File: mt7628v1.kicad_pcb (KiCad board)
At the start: 4 copper layers, 62 x 50.1 mm, 142 parts, among them U1 W9725G6KB-25, U3 W25Q32JVSS, Y1 Crystal_40Mhz

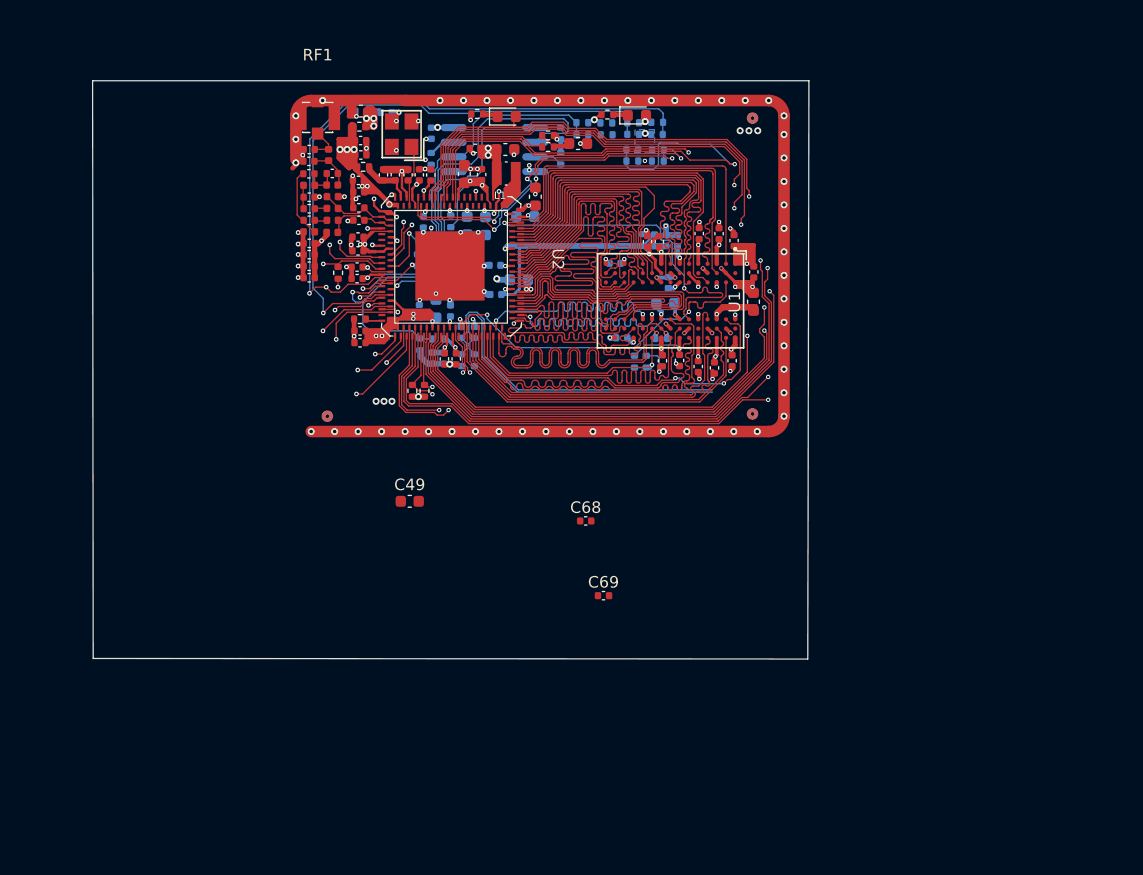
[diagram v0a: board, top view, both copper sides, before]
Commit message: final_all_router by asif
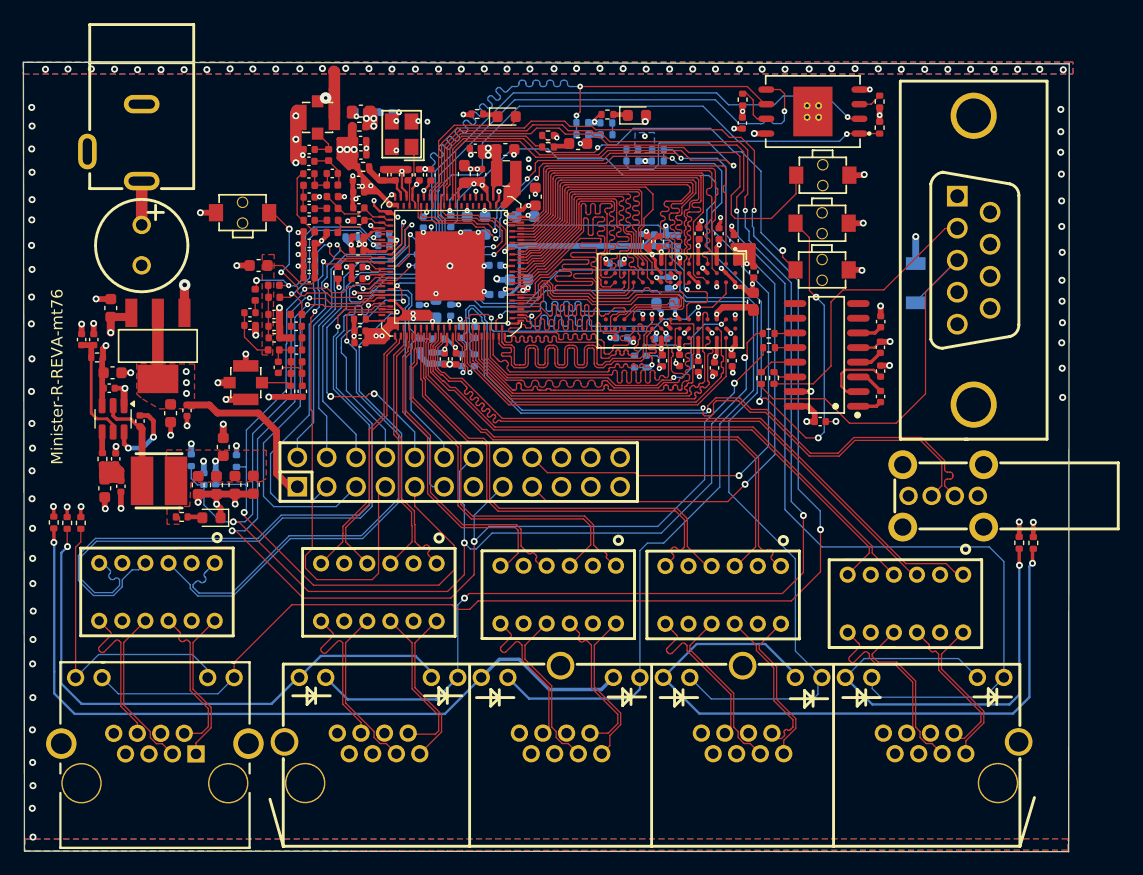
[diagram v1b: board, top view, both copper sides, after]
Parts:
- removed ? (x14): , 
- removed C68: 1uf/6.3v, Capacitor_SMD:C_0402_1005Metric
- removed R15, R16: 10K/1% NC, Resistor_SMD:R_0402_1005Metric
- added C100: 10pf/50v, Capacitor_SMD:C_0402_1005Metric, F.Cu at (117.6, 111.2)
- added C101: 10pf/50v, Capacitor_SMD:C_0402_1005Metric, F.Cu at (113.6, 110.1)
- added C102: 1.2pf/50v, Capacitor_SMD:C_0402_1005Metric, F.Cu at (113.6, 111.2)
- added C103: 1.2pf/50v, Capacitor_SMD:C_0402_1005Metric, F.Cu at (117.7, 113.3)
- added C104: 9pf/50v, Capacitor_SMD:C_0402_1005Metric, F.Cu at (116.1, 114.8)
- added C105: 1.8Pf/50v, Capacitor_SMD:C_0402_1005Metric, F.Cu at (118.2, 116.9)
- added C106: 1.8Pf/50v, Capacitor_SMD:C_0402_1005Metric, F.Cu at (117.1, 116.9)
- added C74: 22uf/25v, Capacitor_SMD:C_0603_1608Metric, F.Cu at (101.6, 109.7)
- added C75: 10uf/6.3v, Capacitor_SMD:C_0603_1608Metric, F.Cu at (106.8, 118.8)
- added C76: 100nf/16v, Capacitor_SMD:C_0402_1005Metric, F.Cu at (108.2, 118.5)
- added C78: 470uf/25v, easyeda2kicad:CAP-TH_BD8.0-P3.50-D0.6-FD, F.Cu at (104.2, 104.2)
- added C79: 2pf/50v, Capacitor_SMD:C_0402_1005Metric, B.Cu at (125.2, 104.3)
- added C80: 2pf/50v, Capacitor_SMD:C_0402_1005Metric, B.Cu at (125.2, 103.3)
- added C81: 1uf/6.3v, Capacitor_SMD:C_0402_1005Metric, F.Cu at (115.7, 112.2)
- added C82: 1uf/6.3v, Capacitor_SMD:C_0402_1005Metric, F.Cu at (115.7, 110.2)
- added C83: 100pf/50v, Capacitor_SMD:C_0402_1005Metric, F.Cu at (115.7, 111.2)
- added C84: 10uf/25v, Capacitor_SMD:C_0603_1608Metric, F.Cu at (101.7, 115.3)
- added C85: 100nf/16v, Capacitor_SMD:C_0402_1005Metric, F.Cu at (101.4, 116.6)
- added C86: NC, Capacitor_SMD:C_0402_1005Metric, F.Cu at (99.0, 112.4)
- added C87: NC, Capacitor_SMD:C_0402_1005Metric, F.Cu at (100.1, 112.4)
- added C88: 1uf/25v, Capacitor_SMD:C_0402_1005Metric, F.Cu at (104.1, 119.5)
- added C89: 22uf/25v, Capacitor_SMD:C_0603_1608Metric, F.Cu at (111.3, 121.7)
- added C90: 22uf/25v, Capacitor_SMD:C_0603_1608Metric, F.Cu at (113.9, 125.0)
- added C91: 22uf/25v, Capacitor_SMD:C_0603_1608Metric, F.Cu at (112.3, 125.0)
- added C92: 22uf/25v, Capacitor_SMD:C_0603_1608Metric, F.Cu at (110.7, 125.0)
- added C93: 22uf/25v, Capacitor_SMD:C_0603_1608Metric, F.Cu at (109.1, 125.0)
- added C94: NC, Capacitor_SMD:C_0402_1005Metric, F.Cu at (102.5, 125.1)
- added C95: 100nf/16v, Capacitor_SMD:C_0402_1005Metric, F.Cu at (168.2, 117.3)
- added C96: 100nf/16v, Capacitor_SMD:C_0402_1005Metric, F.Cu at (168.2, 113.1)
- added C97: 100nf/16v, Capacitor_SMD:C_0402_1005Metric, F.Cu at (168.2, 110.8)
- added C98: 100nf/16v, Capacitor_SMD:C_0402_1005Metric, F.Cu at (163.0, 119.5)
- added C99: 100nf/16v, Capacitor_SMD:C_0402_1005Metric, F.Cu at (168.2, 115.1)
- added D3: LED, Diode_SMD:D_0603_1608Metric, F.Cu at (110.3, 127.8)
- added D4: ZMM5V1, easyeda2kicad:LL-34_L3.5-W1.5-RD, B.Cu at (171.2, 107.5)
- added J1: Barrel_Jack_Switch, easyeda2kicad:DC-IN-TH_DC-005C-20A, F.Cu at (101.9, 95.4)
- added J2: DE9_Pins, easyeda2kicad:HDR-TH_HL-DP9HB180F, F.Cu at (176.3, 105.5)
- added J3: Conn_01x24_MountingPin, easyeda2kicad:HDR-TH_24P-P2.54-V-M-R2-C12-S2.54, F.Cu at (131.7, 123.9)
- added J4: RJ45_LED_Shielded_x2, easyeda2kicad:RJ45-TH_DS1128-09-S8B8X, F.Cu at (105.4, 145.0)
- added L10: 10nh, Inductor_SMD:L_0402_1005Metric, F.Cu at (115.7, 108.7)
- added L11: 6.8uh, easyeda2kicad:IND-SMD_L4.5-W4.0_GCD43-XX, F.Cu at (105.8, 124.6)
- added L12: 10nh, Inductor_SMD:L_0402_1005Metric, F.Cu at (115.7, 107.7)
- added L13: 2nh, Inductor_SMD:L_0402_1005Metric, F.Cu at (117.6, 110.2)
- added L14: 2nh, Inductor_SMD:L_0402_1005Metric, F.Cu at (114.1, 108.5)
- added L15: 2.7nh, Inductor_SMD:L_0402_1005Metric, F.Cu at (117.6, 112.2)
- added L16: 2.7nh, Inductor_SMD:L_0402_1005Metric, F.Cu at (115.7, 113.3)
- added L17: 1.2nh, Inductor_SMD:L_0402_1005Metric, F.Cu at (117.7, 114.3)
- added L18: 2nh, Inductor_SMD:L_0402_1005Metric, F.Cu at (117.6, 115.3)
- added R39: 510/0402, Resistor_SMD:R_0402_1005Metric, F.Cu at (107.7, 127.8)
- added R40: 1k/1%, Resistor_SMD:R_0402_1005Metric, F.Cu at (97.8, 128.3)
- added R41: 1k/1%, Resistor_SMD:R_0402_1005Metric, F.Cu at (96.6, 128.2)
- added R42: 1k/1%, Resistor_SMD:R_0402_1005Metric, F.Cu at (181.4, 130.0)
- added R43: 1k/1%, Resistor_SMD:R_0402_1005Metric, F.Cu at (180.2, 130.0)
- added R44: 1k/1%, Resistor_SMD:R_0402_1005Metric, F.Cu at (99.0, 128.3)
- added R46: 100K/0402, Resistor_SMD:R_0402_1005Metric, F.Cu at (100.4, 114.0)
- added R47: 1k/1%, Resistor_SMD:R_0402_1005Metric, F.Cu at (100.8, 122.7)
- added R48: 6.2K/0603, Capacitor_SMD:C_0603_1608Metric, F.Cu at (101.0, 125.3)
- added R49: 2K/0402, Capacitor_SMD:C_0402_1005Metric, F.Cu at (102.0, 122.7)
- added R50: 0, Resistor_SMD:R_0402_1005Metric, F.Cu at (158.5, 111.9)
- added R52: 0, Resistor_SMD:R_0402_1005Metric, F.Cu at (158.6, 113.1)
- added R55: 0, Resistor_SMD:R_0402_1005Metric, F.Cu at (157.9, 115.7)
- added R57: 0, Resistor_SMD:R_0402_1005Metric, F.Cu at (159.0, 115.7)
- added RF2: ANT_SHAFT_SEAT, easyeda2kicad:IPEX-SMD_4P-L2.6-W2.6_C9900016457, F.Cu at (113.3, 116.1)
- added SW_GPIO1: GPIO, easyeda2kicad:SW-SMD_L3.9-W2.9-LS4.8-EH-A, F.Cu at (113.0, 101.4)
- added SW_GPIO3: PORST, easyeda2kicad:SW-SMD_L3.9-W2.9-LS4.8-EH-A, F.Cu at (163.1, 106.4)
- added SW_REF_CLK1: REF_CLK, easyeda2kicad:SW-SMD_L3.9-W2.9-LS4.8-EH-A, F.Cu at (163.2, 98.2)
- added SW_WDT_RST1: WDT_RST, easyeda2kicad:SW-SMD_L3.9-W2.9-LS4.8-EH-A, F.Cu at (163.1, 102.3)
- added U10: ~, easyeda2kicad:RJ45-TH_B-1-4, F.Cu at (148.4, 144.4)
- added U11: TF-1016DG-LAN3, easyeda2kicad:DIP-12_L12.8-W7.3-P2.00-LS5.0-BL, F.Cu at (140.3, 134.5)
- added U12: TF-1016DG-LAN2, easyeda2kicad:DIP-12_L12.8-W7.3-P2.00-LS5.0-BL, F.Cu at (154.6, 134.5)
- added U13: TF-1016DG-LAN1, easyeda2kicad:DIP-12_L12.8-W7.3-P2.00-LS5.0-BL, F.Cu at (170.3, 135.2)
- added U14: TF-1016DG-WAN, easyeda2kicad:DIP-12_L12.8-W7.3-P2.00-LS5.0-BL, F.Cu at (105.6, 134.2)
- added U4: ams1117-5v, easyeda2kicad:SOT-223_L6.5-W3.5-P2.30-LS7.0-BR, F.Cu at (105.7, 113.0)
- added U6: TF-1016DG-LAN4, easyeda2kicad:DIP-12_L12.8-W7.3-P2.00-LS5.0-BL, F.Cu at (124.8, 134.3)
- added U7: MP1470, Package_TO_SOT_SMD:TSOT-23-6, F.Cu at (101.8, 119.3)
- added U8: SP3232, easyeda2kicad:SOIC-16_L9.9-W3.9-P1.27-LS6.0-BL, F.Cu at (163.5, 113.7)
- added U9: USB_VERTICLE, easyeda2kicad:USB-A-TH_USB-226-BRW, F.Cu at (173.6, 125.9)
- C69: moved to B.Cu
- C70, R22, R23, R24: moved to F.Cu
- L1: value 2.2 uH/VLS252012T-2R2M1R3 -> 2.2 uH/VLS252012ET-2R2M; footprint Library:IND_VLS252012ET-100M -> easyeda2kicad:IND-SMD_L2.5-W2.0_VLS2520X
- U1: value W9725G6KB-25 -> W971GG6SB25I; footprint easyeda2kicad:WBGA-84_L12.5-W8.0-P0.80-TL_WINBOND_W9725G6KB -> easyeda2kicad:WBGA-84_L12.5-W8.0-P0.80-TL_W9751G6KB
- U2: value ~ -> MT7628NN
- U3: value W25Q32JVSS -> W25Q256JVEIQ; footprint easyeda2kicad:SOIC-8_L5.3-W5.3-P1.27-LS8.0-BL -> easyeda2kicad:WSON-8_L8.0-W6.10-P1.27-BL-EP; moved to F.Cu
- moved R5 48.4 mm to (110.7, 124.4), turned to -90 degrees
- moved R29 48.1 mm to (108.5, 122.8), turned to -90 degrees
- moved R28 47.7 mm to (109.6, 124.5), turned to -90 degrees
- moved R6 46.7 mm to (112.5, 122.9), turned to -90 degrees
- moved C69 38.0 mm to (122.4, 103.5), turned to 180 degrees
- moved R22 28.0 mm to (168.1, 91.8), turned to 90 degrees
- moved U3 27.8 mm to (162.3, 92.7), turned to 90 degrees
- moved R23 27.6 mm to (168.1, 94.1), turned to 90 degrees
- moved R24 27.4 mm to (156.3, 91.6)
- moved C70 26.9 mm to (156.2, 93.7)
- moved C49 24.2 mm to (114.4, 106.0), turned to 180 degrees
- moved R17 0.06 mm to (131.0, 109.9)
- moved C32 0.05 mm to (134.0, 102.5)
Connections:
- net Net-(U2C-WDT_RST_N) renamed WDT_RST
- net Net-(U2D-USB_DM) renamed USB_DP-
- net Net-(U2D-USB_DP) renamed USB_DP+
- U1 pad R8: MADDR13 -> unconnected-(U1-A13(2GB)-PadR8)
- U2 pad 11: unconnected-(U2A-WF1_RFION-Pad11) -> WF1_RF1ON
- U2 pad 12: unconnected-(U2A-WF1_RFIOP-Pad12) -> WF1_RF1OP
- U2 pad 138: PORST_N -> CPURST_N
- U2 pad 139: WIFI_RESET -> LINK4
- U2 pad 140: unconnected-(U2E-AVDD33_TX_P1234_2-Pad140) -> LINK3
- U2 pad 141: unconnected-(U2E-EPHY_LED2_N_JTMS-Pad141) -> LINK2
- U2 pad 142: EPH_LED1_N -> LINK1
- U2 pad 143: EPH_LED0_N -> LINK0
- U2 pad 16: I2S_DI -> I2S_SDI
- U2 pad 17: I2S_D0 -> I2S_SDO
- U2 pad 40: TXOP1 -> RXN1
- U2 pad 42: TXON1 -> RXP1
- U2 pad 43: RXIP1 -> TXN1
- U2 pad 44: RXIN1 -> TXP1
- U2 pad 45: PWM_CH0 -> RXN2
- U2 pad 46: PWM_CH1 -> RXP2
- U2 pad 47: UART_RXD2 -> TXN2
- U2 pad 48: UART_TXD2 -> TXP2
- U2 pad 49: SD_WP -> RXN3
- U2 pad 50: SD_CD -> RXP3
- U2 pad 51: SD_D1 -> TXN3
- U2 pad 52: SD_D0 -> TXP3
- U2 pad 54: SD_CLK -> RXN4
- U2 pad 55: SD_CMD -> RXP4
- U2 pad 56: SD_D3 -> TXN4
- U2 pad 57: SD_D2 -> TXP4
- U2 pad 7: unconnected-(U2A-AVSS33_RF_3-Pad7) -> GND
- U2 pad 83: MADDR13 -> unconnected-(U2B-MA13-Pad83)
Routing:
- net LINK0: track 0.00 -> 141.8 mm, vias 0 -> 2
- net LINK1: track 0.00 -> 121.8 mm, vias 0 -> 3
- net LINK4: track 0.00 -> 109.5 mm, vias 0 -> 1
- net UART_RXD0: track 4.38 -> 98.2 mm, vias 1 -> 4
- net LINK3: track 0.00 -> 92.6 mm, vias 0 -> 1
- net LINK2: track 0.00 -> 90.3 mm, vias 0 -> 1
- net WDT_RST: track 0.46 -> 75.1 mm, vias 1 -> 4
- net /ethernet/12: track 0.00 -> 66.9 mm, vias 0 -> 1
- net SPI_CLK: track 26.0 -> 88.0 mm, vias 0 -> 4
- net /ethernet/13: track 0.00 -> 60.6 mm, vias 0 -> 1
- net UART_TXD0: track 52.3 -> 110.8 mm, vias 1 -> 4
- net RXIP0: track 1.11 -> 59.5 mm
- net TXP4: track 0.00 -> 56.7 mm
- net TXN4: track 0.00 -> 56.6 mm
- net GND: track 201.1 -> 145.6 mm, vias 131 -> 201
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- added copper zone on In2.Cu, net +12V
- added copper zone on F.Cu, net +5V
- added copper zone on F.Cu, net 3.3VD
- added copper zone on F.Cu, net 3.3V_RF
- added copper zone on B.Cu, net GND
- added copper zone on F.Cu, net GND
- added copper zone on In2.Cu, net GND
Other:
- board size 62 x 50.1 mm -> 90.5 x 68.3 mm
- board text added: "Developed by"
- board text added: "Intricate Technology"
- board text added: "Minister-R-REVA-mt76"
